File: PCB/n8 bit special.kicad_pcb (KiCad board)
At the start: 2 copper layers, 35 parts, among them J1 PowerPort, J2 PORT0, J3 PORT2, J4 PORT1, J5 PORT3, J6 Conn_02x08_Odd_Even, SW1 SW_Push_Dual, U1 W65C02SxP, U2 74LS21, U3 DS1813, U4 22V10C, U5 CY62256-70PC, U6 CY62256-70PC, U7 28C256, X1 2Mhz

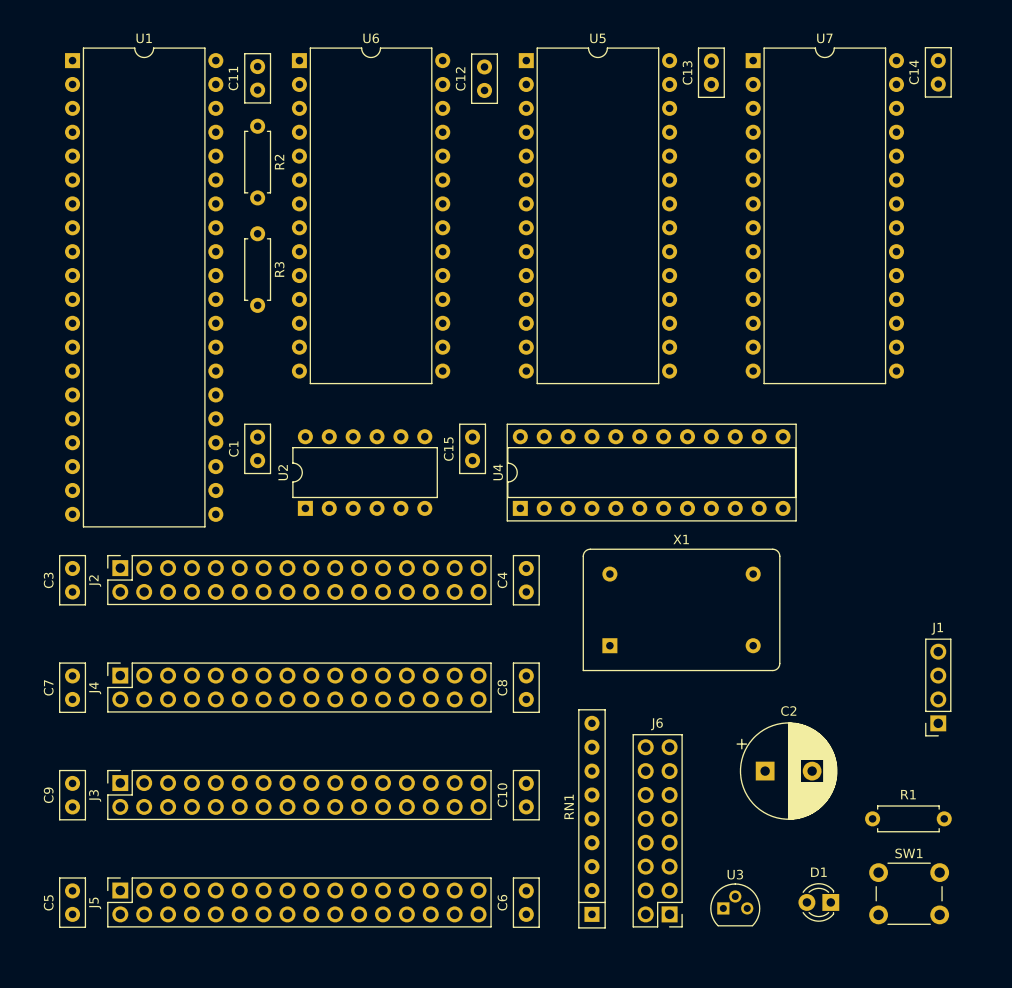
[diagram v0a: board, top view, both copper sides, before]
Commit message: Near final board
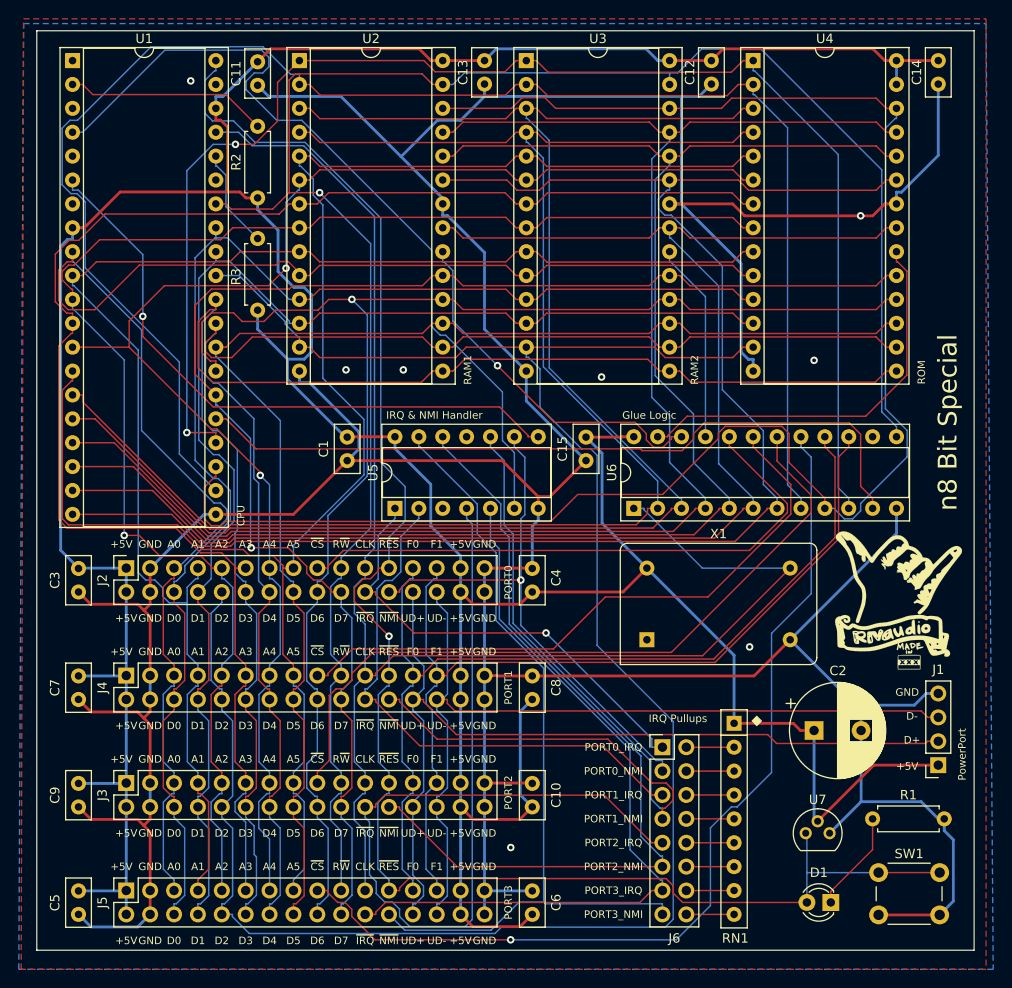
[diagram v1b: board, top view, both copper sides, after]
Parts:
- removed the U6 at (114.9, 45.1)
- added G***: LOGO, graphics:Shaka, F.Cu at (178.6, 101.9)
- added U4: 28C256, Package_DIP:DIP-28_W15.24mm_Socket, F.Cu at (163.2, 45.1)
- U1: footprint Package_DIP:DIP-40_W15.24mm -> Package_DIP:DIP-40_W15.24mm_Socket
- U2: value 74LS21 -> CY62256-70PC; footprint Package_DIP:DIP-12_W7.62mm -> Package_DIP:DIP-28_W15.24mm_Socket
- U3: value DS1813 -> CY62256-70PC; footprint Package_TO_SOT_THT:TO-92 -> Package_DIP:DIP-28_W15.24mm_Socket
- U5: value CY62256-70PC -> 74LS21; footprint Package_DIP:DIP-28_W15.24mm -> Package_DIP:DIP-14_W7.62mm_Socket
- U7: value 28C256 -> DS1813; footprint Package_DIP:DIP-28_W15.24mm -> Package_TO_SOT_THT:TO-92
- moved U3 92.6 mm to (139.1, 45.1)
- moved U7 82.4 mm to (168.8, 127.3)
- moved U5 49.6 mm to (125.1, 92.7), turned to 90 degrees
- moved U2 47.6 mm to (114.9, 45.1), turned to 0 degrees
- moved RN1 25.3 mm to (161.2, 115.6), turned to 270 degrees
- moved C12 24.3 mm to (158.8, 45.1), turned to 270 degrees
- moved C13 24.3 mm to (134.6, 45.1), turned to 270 degrees
- moved J6 17.8 mm to (153.5, 118.1), turned to 0 degrees
- moved C15 12.1 mm to (145.4, 87.6)
- moved U6 12.1 mm to (150.5, 92.7)
- moved C1 9.53 mm to (120.0, 87.6)
- moved C2 6.76 mm to (169.7, 116.3)
- moved J1 4.45 mm to (182.9, 120.0)
- moved X1 3.99 mm to (151.9, 106.7)
- moved C10 0.63 mm to (139.7, 124.5)
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- renumbered U4 to U6
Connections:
- U2 pad 1: PORT0_IRQ_PULLUP -> /A14
- U2 pad 10: PORT1_NMI_PULLUP -> /A0
- U2 pad 11: (no net) -> /D0
- U2 pad 12: PORT2_NMI_PULLUP -> /D1
- U2 pad 2: PORT1_IRQ_PULLUP -> /A12
- U2 pad 3: (no net) -> /A7
- U2 pad 4: PORT2_IRQ_PULLUP -> /A6
- U2 pad 5: PORT3_IRQ_PULLUP -> /A5
- U2 pad 6: ~IRQ -> /A4
- U2 pad 7: GND -> /A3
- U2 pad 8: ~NMI -> /A2
- U2 pad 9: PORT0_NMI_PULLUP -> /A1
- U3 pad 1: ~RES -> /A14
- U3 pad 2: +5V -> /A12
- U3 pad 3: GND -> /A7
- U5 pad 1: /A14 -> PORT0_IRQ_PULLUP
- U5 pad 10: /A0 -> PORT1_NMI_PULLUP
- U5 pad 11: /D0 -> (no net)
- U5 pad 12: /D1 -> PORT2_NMI_PULLUP
- U5 pad 13: /D2 -> PORT3_NMI_PULLUP
- U5 pad 14: GND -> +5V
- U5 pad 2: /A12 -> PORT1_IRQ_PULLUP
- U5 pad 3: /A7 -> (no net)
- U5 pad 4: /A6 -> PORT2_IRQ_PULLUP
- U5 pad 5: /A5 -> PORT3_IRQ_PULLUP
- U5 pad 6: /A4 -> ~IRQ
- U5 pad 7: /A3 -> GND
- U5 pad 8: /A2 -> ~NMI
- U5 pad 9: /A1 -> PORT0_NMI_PULLUP
- U7 pad 1: /A14 -> ~RES
- U7 pad 2: /A12 -> +5V
- U7 pad 3: /A7 -> GND
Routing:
- net GND: track 0.00 -> 483.3 mm, vias 0 -> 8
- net +5V: track 0.00 -> 438.1 mm
- net /D2: track 0.00 -> 218.0 mm
- net R~W: track 0.00 -> 205.8 mm, vias 0 -> 1
- net /A13: track 0.00 -> 184.3 mm
- net /A5: track 0.00 -> 180.0 mm
- net ~RES: track 0.00 -> 177.3 mm, vias 0 -> 1
- net /A12: track 0.00 -> 174.3 mm
- net /A7: track 0.00 -> 170.6 mm
- net /A11: track 0.00 -> 169.3 mm
- net /A3: track 0.00 -> 167.5 mm
- net /A0: track 0.00 -> 166.3 mm
- net /A9: track 0.00 -> 166.0 mm
- net /A8: track 0.00 -> 166.0 mm
- net /A6: track 0.00 -> 165.7 mm
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- added copper zone on B.Cu, net GND
- added copper zone on F.Cu, net GND
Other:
- board outline added: 99.7 x 97.8 mm
- net class Default: trace_width 0.25 -> 0.154
- net class Power added: clearance 0.3, trace_width 0.3, via_dia 0.8, via_drill 0.4
- rule trace_min: 0.2 -> 0.154
- board text added: "+5V"
- board text added: "A0"
- board text added: "A1"
- board text added: "A2"
- board text added: "A3"
- board text added: "A4"
- board text added: "A5"
- board text added: "CLK"
- board text added: "CPU"
- board text added: "D+"
- board text added: "D-"
- board text added: "D0"
- board text added: "D1"
- board text added: "D2"
- board text added: "D3"
- board text added: "D4"
- board text added: "D5"
- board text added: "D6"
- board text added: "D7"
- board text added: "F0"
- board text added: "F1"
- board text added: "GND"
- board text added: "Glue Logic"
- board text added: "IRQ & NMI Handler"
- board text added: "IRQ Pullups"
- board text added: "PORT0"
- board text added: "PORT0_IRQ"
- board text added: "PORT0_NMI"
- board text added: "PORT1"
- board text added: "PORT1_IRQ"
- board text added: "PORT1_NMI"
- board text added: "PORT2"
- board text added: "PORT2_IRQ"
- board text added: "PORT2_NMI"
- board text added: "PORT3"
- board text added: "PORT3_IRQ"
- board text added: "PORT3_NMI"
- board text added: "PowerPort"
- board text added: "RAM1"
- board text added: "RAM2"
- board text added: "ROM"
- board text added: "R~W"
- board text added: "UD+"
- board text added: "UD-"
- board text added: "by Nate Rivard https://github.com/nrivard/lmaos Version 1 Mar 2021"
- board text added: "n8 Bit Special"
- board text added: "~CS"
- board text added: "~IRQ"
- board text added: "~NMI"
- board text added: "~RES"
